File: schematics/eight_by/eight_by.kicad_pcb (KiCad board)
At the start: 2 copper layers, 172.7 x 44.4 mm, 42 parts, among them J1 Conn_01x08, SW1 SW_Push_45deg, SW2 SW_Push_45deg, SW3 SW_Push_45deg, SW4 SW_Push_45deg, SW5 SW_Push_45deg, SW6 SW_Push_45deg, SW7 SW_Push_45deg, SW8 SW_Push_45deg, U1 74HC4051, U2 74HC4051

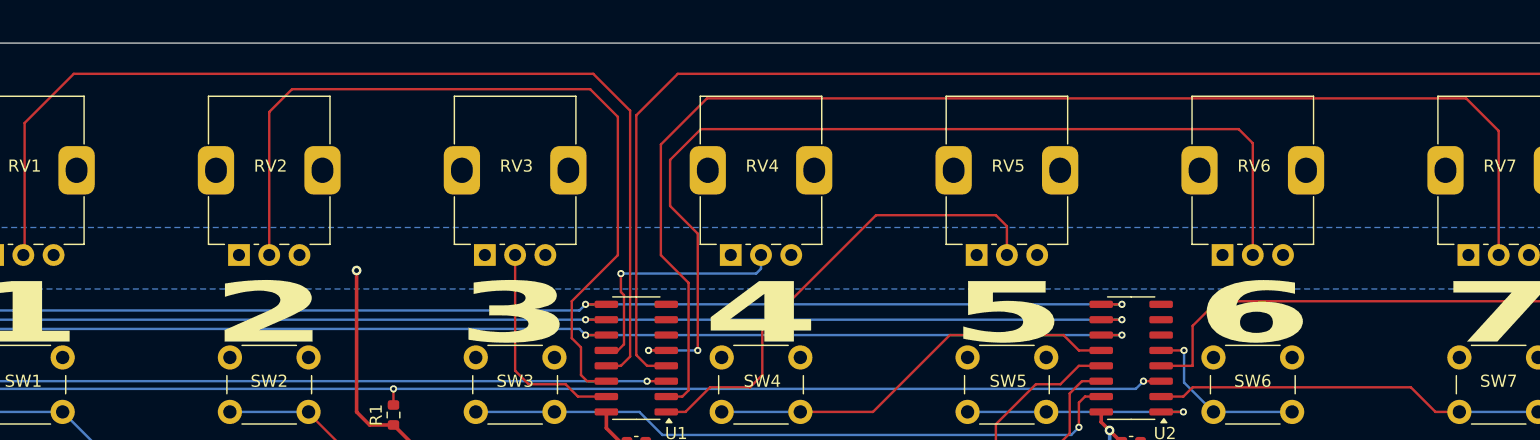
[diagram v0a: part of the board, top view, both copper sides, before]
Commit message: eight_by_qtpy idea
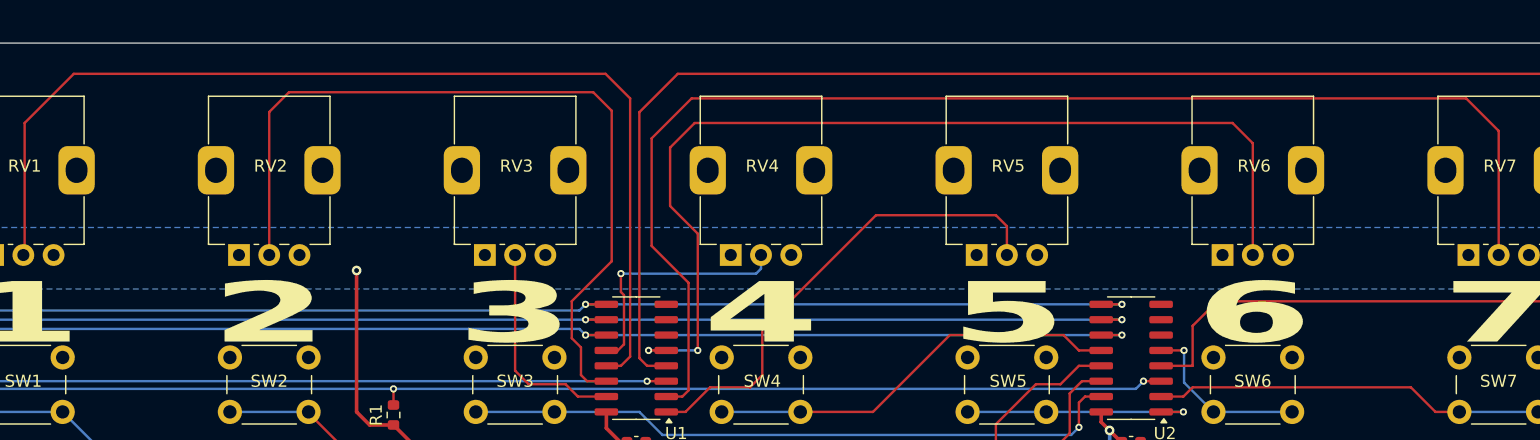
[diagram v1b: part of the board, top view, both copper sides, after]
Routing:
- net /POT7: track 105.5 -> 106.9 mm
- net /POT6: track 81.1 -> 82.2 mm
- net /POT2: track 67.9 -> 67.3 mm
- net /POT1: track 87.4 -> 88.0 mm
